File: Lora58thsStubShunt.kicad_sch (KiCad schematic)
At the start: 11 parts, among them J1 Conn_Coaxial, J2 Conn_01x01_Pin, J3 Conn_01x01_Pin, J4 Conn_01x01_Pin

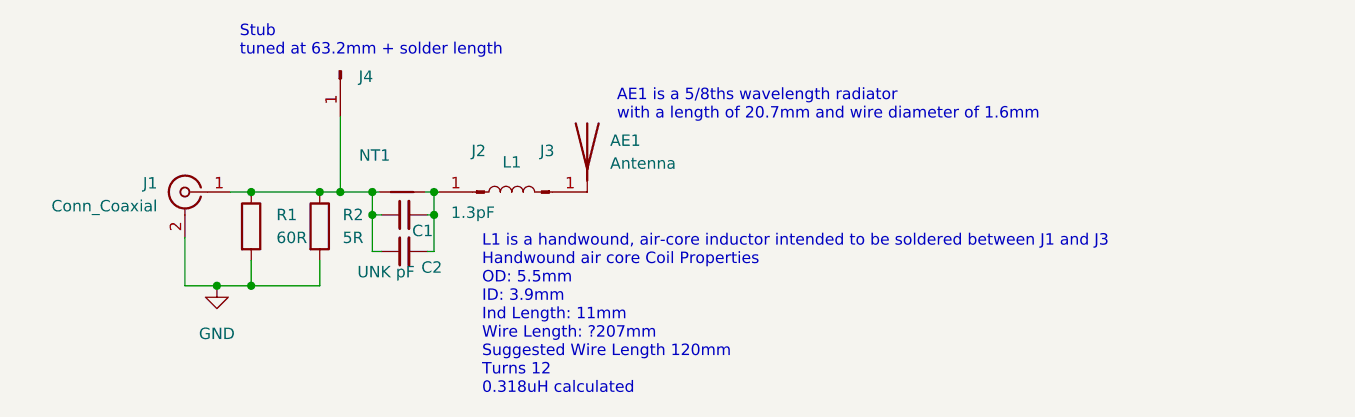
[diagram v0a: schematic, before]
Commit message: Release Candidate
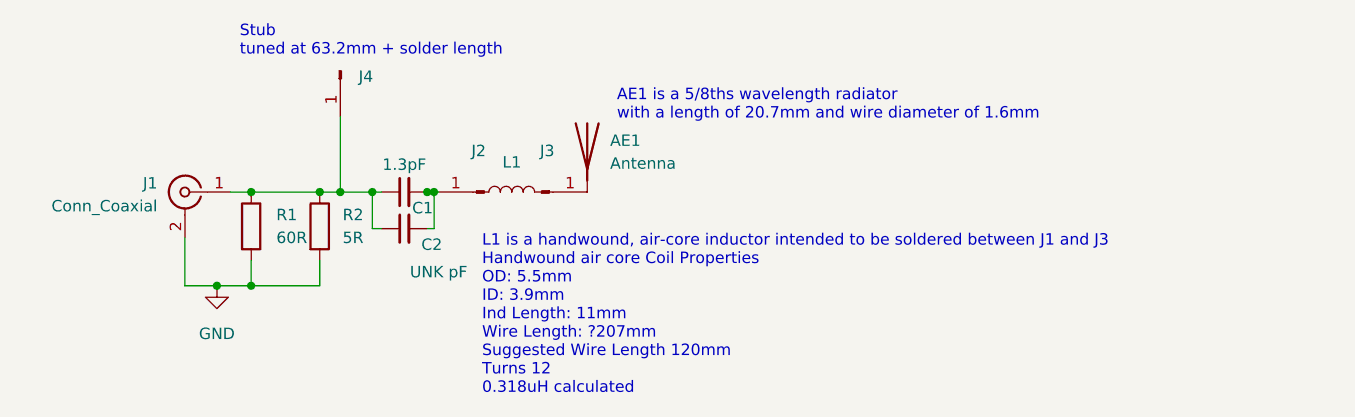
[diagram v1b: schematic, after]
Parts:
- removed NT1: NetTie_2, Jumper:SolderJumper-2_P1.3mm_Open_RoundedPad1.0x1.5mm, symbol Device:NetTie_2
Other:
- moved on the sheet: C1, C2
